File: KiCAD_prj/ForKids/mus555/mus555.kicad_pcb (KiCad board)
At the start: 2 copper layers, 83.8 x 45.8 mm, 24 parts, among them J1 Screw_Terminal_01x02, SW1 SW_Push, SW2 SW_Push, SW3 SW_Push, SW4 SW_Push, SW5 SW_Push, SW6 SW_Push, SW7 SW_Push, SW8 SW_Push, U1 NE555

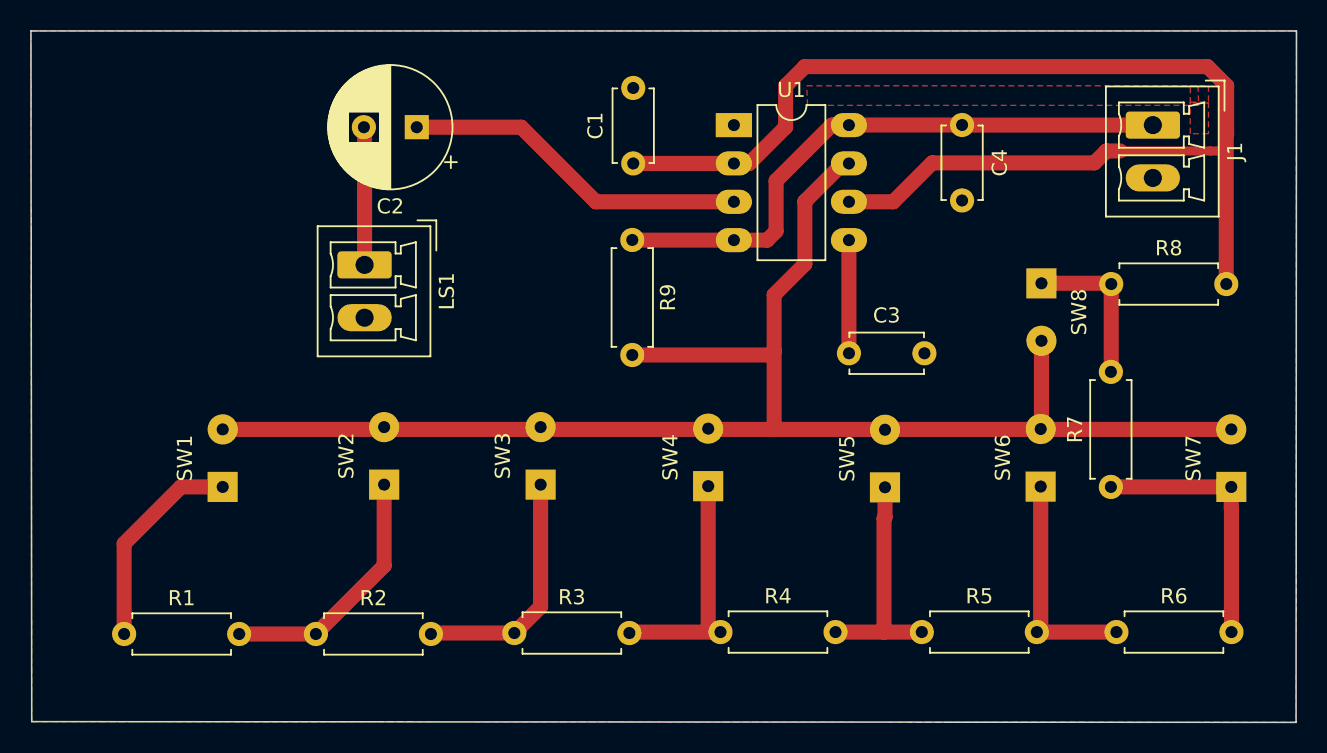
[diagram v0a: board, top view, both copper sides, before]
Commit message: Update files KiCAD mus555 zip
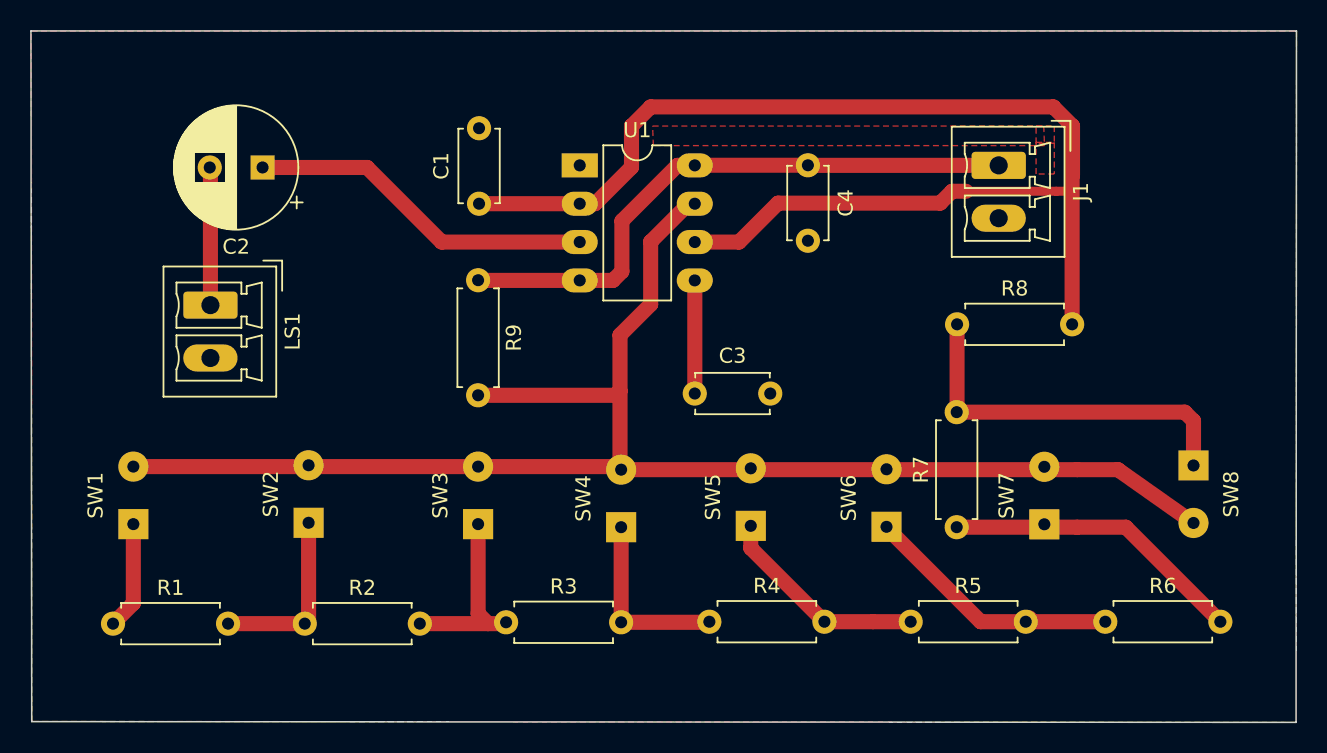
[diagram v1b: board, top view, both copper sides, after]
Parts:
- moved SW8 15.7 mm to (76.9, -17.0)
- moved SW7 12.6 mm to (67.1, -13.1)
- moved J1 10.6 mm to (64.0, -36.8)
- moved R8 10.6 mm to (61.3, -26.3)
- moved R9 10.6 mm to (29.6, -29.2)
- moved LS1 10.6 mm to (11.8, -27.6)
- moved C1 10.6 mm to (29.6, -34.3)
- moved C3 10.6 mm to (43.9, -21.7)
- moved C4 10.6 mm to (51.4, -36.8)
- moved R7 10.6 mm to (61.3, -12.9)
- moved SW6 10.6 mm to (56.6, -12.9)
- moved U1 10.6 mm to (36.3, -36.8)
- moved C2 10.6 mm to (15.3, -36.7)
- moved SW5 9.25 mm to (47.6, -13.0)
- moved SW1 6.41 mm to (6.73, -13.1)
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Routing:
- net Net-(R7-Pad2): track 10.6 -> 24.9 mm
- net Net-(R1-Pad1): track 14.1 -> 7.15 mm
- net Net-(R1-Pad2): track 16.8 -> 11.9 mm
- net Net-(R3-Pad2): track 15.8 -> 12.2 mm
- net Net-(R2-Pad2): track 16.1 -> 12.7 mm
- net Net-(R5-Pad2): track 15.1 -> 17.6 mm
- net Net-(R6-Pad2): track 17.5 -> 20.0 mm
- net Net-(R9-Pad2): track 102.3 -> 100.8 mm
- net Net-(R4-Pad2): track 15.3 -> 14.1 mm
